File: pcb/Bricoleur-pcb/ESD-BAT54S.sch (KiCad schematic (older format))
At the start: 1 part

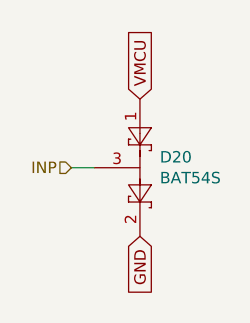
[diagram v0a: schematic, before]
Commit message: Moar routing
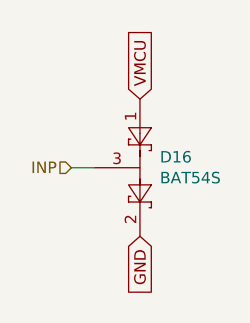
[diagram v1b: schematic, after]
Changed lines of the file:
@@
 AR Path="/5BEE7FFD/5BEC0258/5BB71F8A" Ref="D19"  Part="1"
 AR Path="/5BEE7FFD/5BEC025B/5BB71F8A" Ref="D20"  Part="1"
-F 0 "D20" V 5804 3037 50  0000 L CNN
+F 0 "D16" V 5804 3037 50  0000 L CNN
 F 1 "BAT54S" V 5895 3037 50  0000 L CNN
 F 2 "Package_TO_SOT_SMD:SOT-23" H 5925 3075 50  0001 L CNN
